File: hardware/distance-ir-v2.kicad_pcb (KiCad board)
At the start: 2 copper layers, 18.9 x 44.6 mm, 25 parts, among them P1 CON-SENSOR2, P2 DEBUG, P3 BOOT, P4 S3B-PH-SM4, U2 DRILL, U3 DRILL, U4 XMC1302

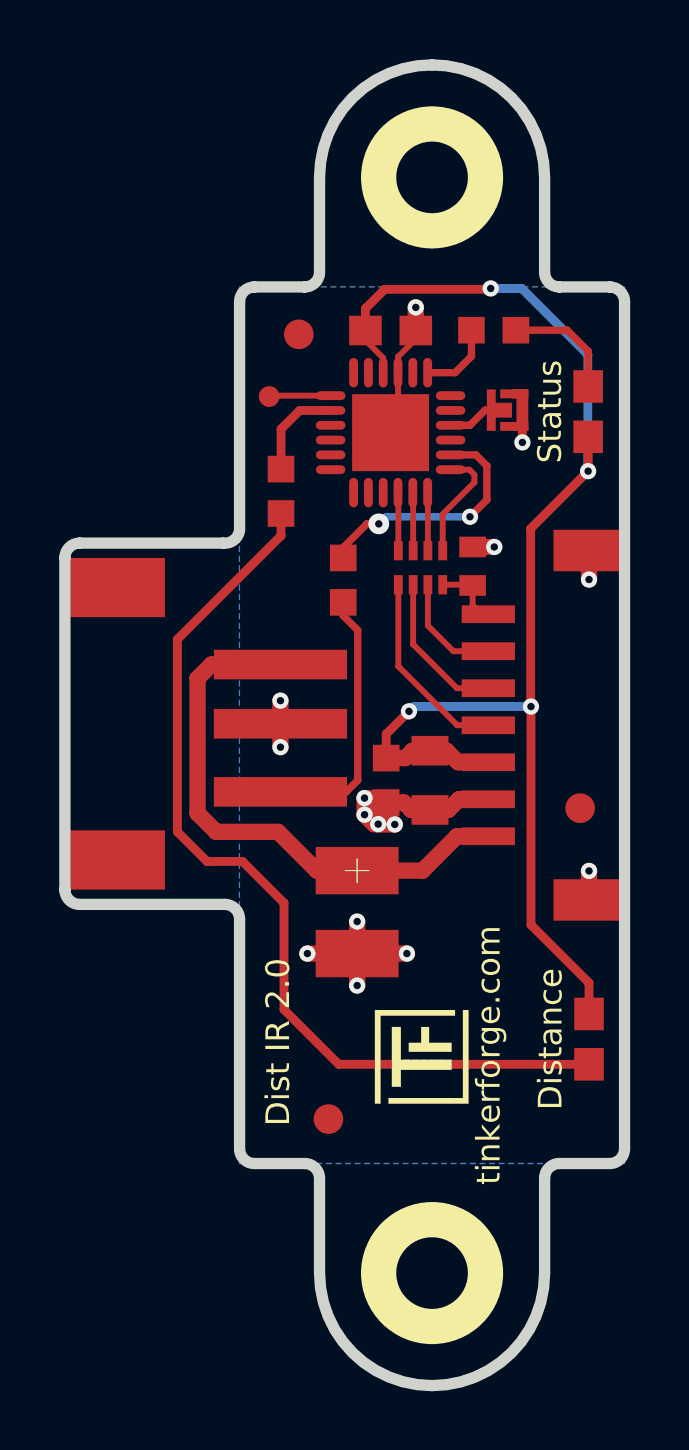
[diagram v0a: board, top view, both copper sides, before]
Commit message: update to new kicad version
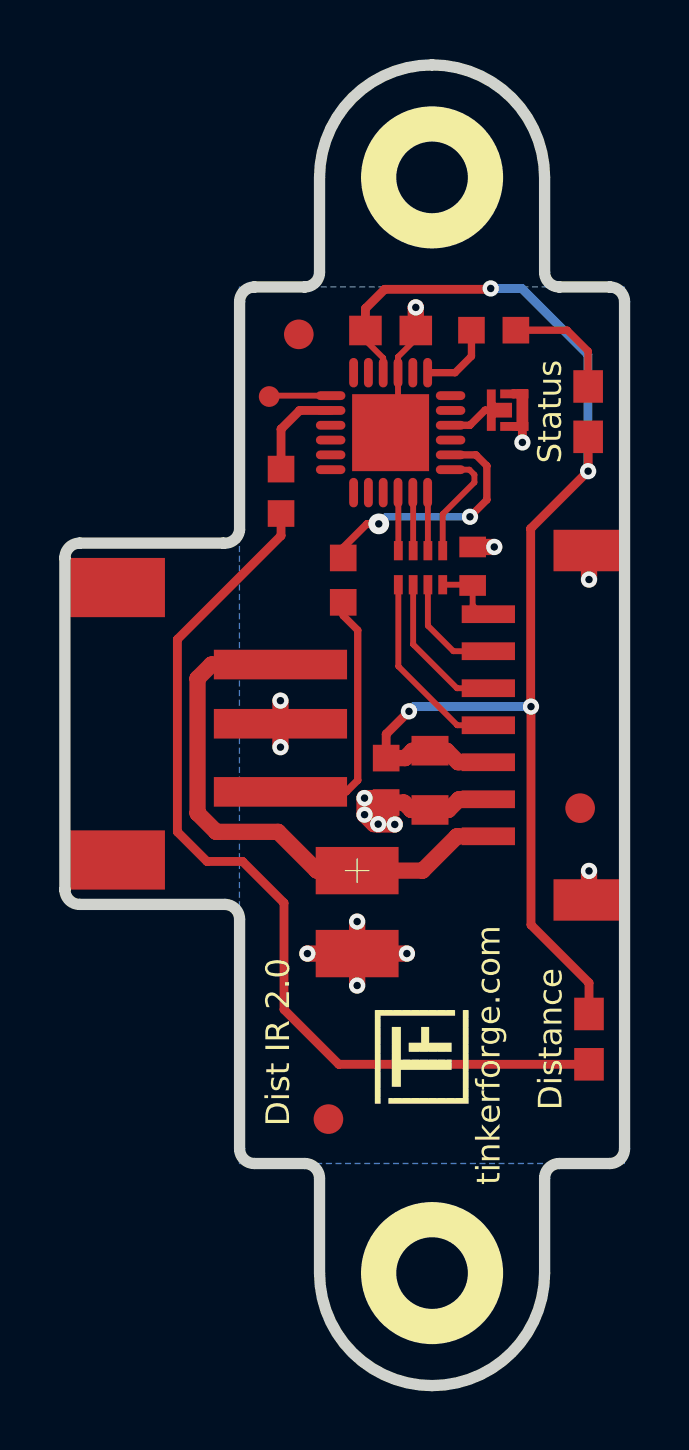
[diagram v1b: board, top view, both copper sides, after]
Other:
- outline, holes or cut-outs redrawn
- net class Default removed
